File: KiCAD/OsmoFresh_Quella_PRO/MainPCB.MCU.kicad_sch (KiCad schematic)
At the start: 14 parts

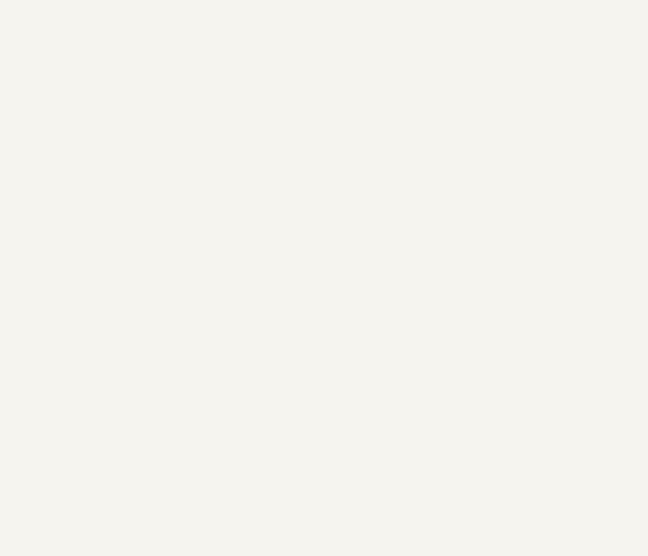
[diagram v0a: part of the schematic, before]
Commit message: Update Schematics
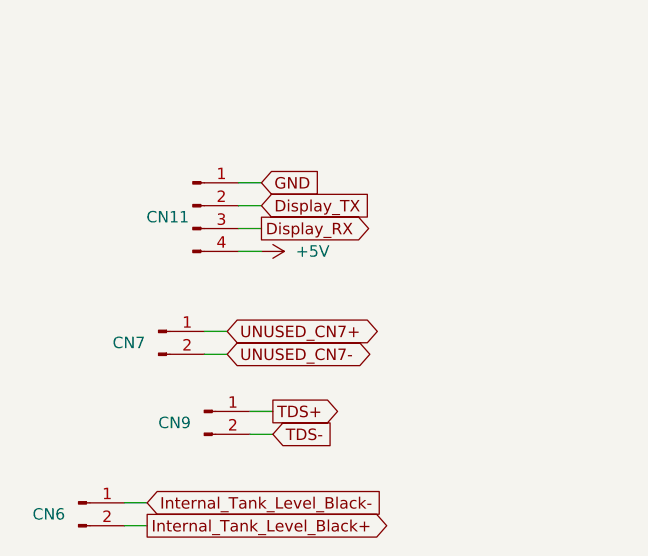
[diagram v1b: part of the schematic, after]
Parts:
- added CN11: Conn_01x04_Pin, symbol Connector:Conn_01x04_Pin
- added CN6, CN7, CN9: Conn_01x02_Pin, symbol Connector:Conn_01x02_Pin
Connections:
- net +5V: now also CN11.4 (Pin_4)
- net Display_RX: now also CN11.3 (Pin_3)
- net Display_TX: now also CN11.2 (Pin_2)
- net GND: now also CN11.1 (Pin_1)
- net Internal_Tank_Level_Black+: now also CN6.2 (Pin_2)
- net TDS+: now also CN9.1 (Pin_1)
- net TDS-: now also CN9.2 (Pin_2)
- net UNUSED_CN7+: now also CN7.1 (Pin_1)
- net UNUSED_CN7-: now also CN7.2 (Pin_2)
- new net Internal_Tank_Level_Black-: CN6.1 (Pin_1)
